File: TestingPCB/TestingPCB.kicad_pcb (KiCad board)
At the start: 2 copper layers, 15 parts, among them J1 Conn_01x04, J2 USB_C_Receptacle_USB2.0_14P, J3 Conn_01x08, U1 SC0915, U2 CP2102N-Axx-xQFN24, U3 USBLC6-2P6

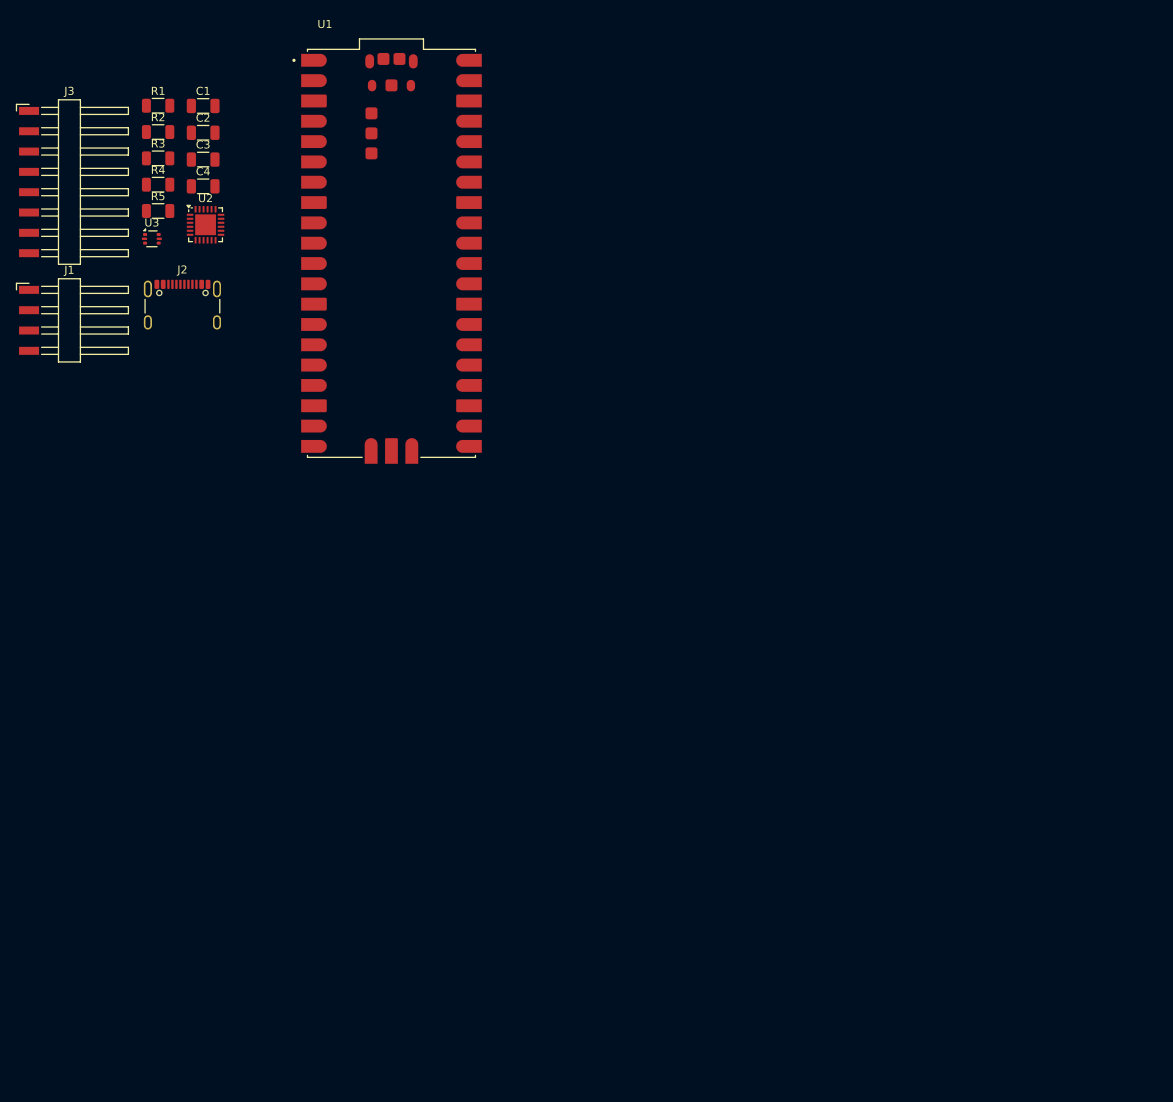
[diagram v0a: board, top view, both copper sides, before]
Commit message: v1 of PCB
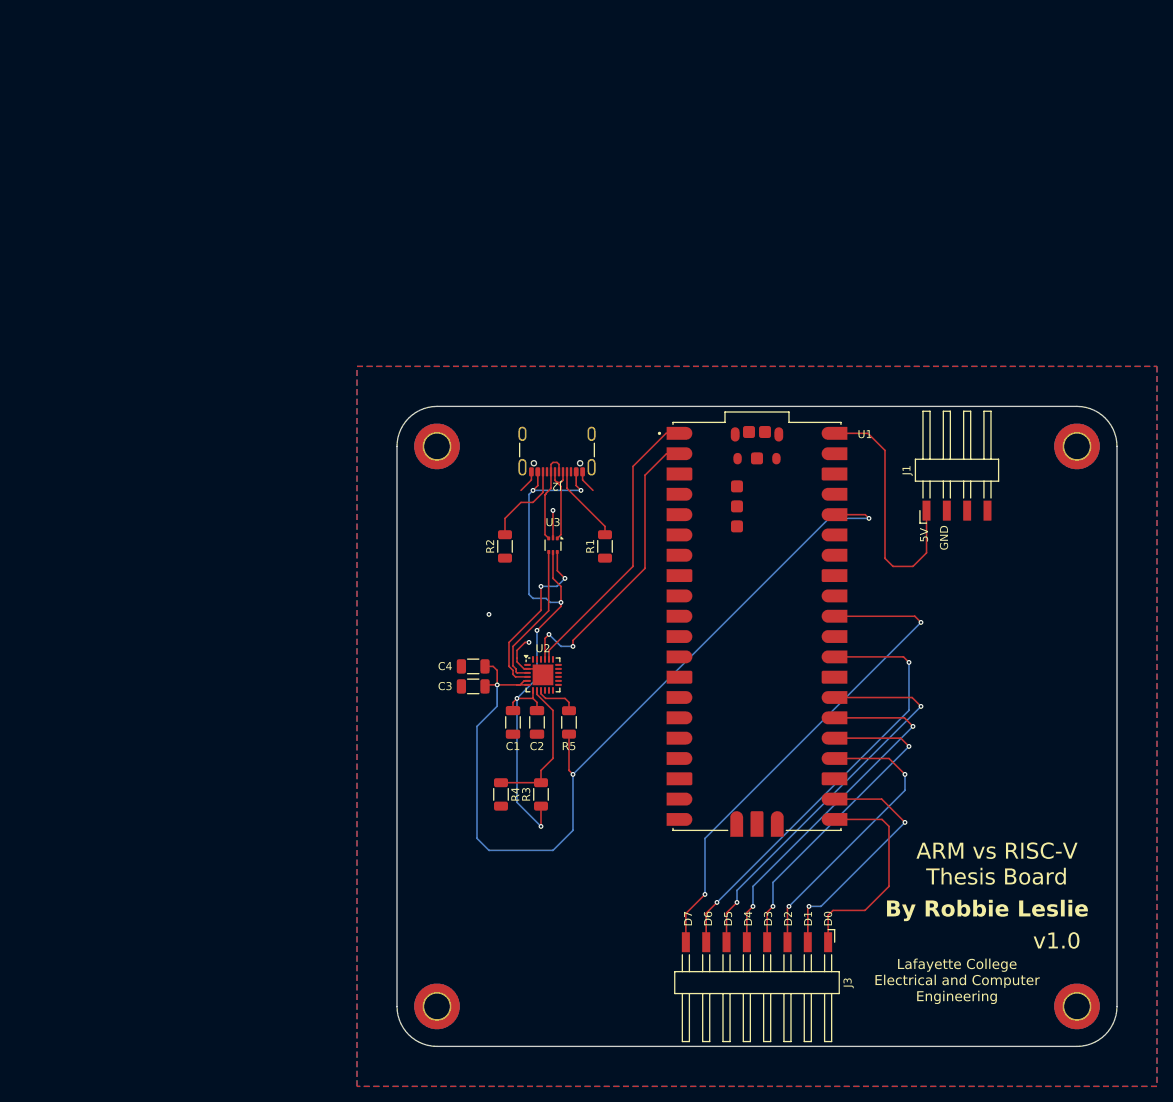
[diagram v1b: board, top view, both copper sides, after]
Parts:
- added H1: MountingHole, MountingHole:MountingHole_3.2mm_M3_ISO7380_Pad_TopBottom, F.Cu at (95.0, 70.0)
- added H2: MountingHole, MountingHole:MountingHole_3.2mm_M3_ISO7380_Pad_TopBottom, F.Cu at (175.0, 70.0)
- added H3: MountingHole, MountingHole:MountingHole_3.2mm_M3_ISO7380_Pad_TopBottom, F.Cu at (95.0, 140.0)
- added H4: MountingHole, MountingHole:MountingHole_3.2mm_M3_ISO7380_Pad_TopBottom, F.Cu at (175.0, 140.0)
- moved J3 132.0 mm to (135.0, 137.5), turned to -90 degrees
- moved J1 112.0 mm to (160.0, 72.5), turned to 90 degrees
- moved R3 92.8 mm to (108.0, 113.5), turned to 90 degrees
- moved R4 87.4 mm to (103.0, 113.5), turned to -90 degrees
- moved C1 86.2 mm to (104.5, 104.5), turned to -90 degrees
- moved C2 84.7 mm to (107.5, 104.5), turned to -90 degrees
- moved R5 82.0 mm to (111.5, 104.5), turned to 90 degrees
- moved R1 78.5 mm to (116.0, 82.5), turned to 90 degrees
- moved C3 74.0 mm to (99.5, 100.0), turned to 180 degrees
- moved U2 70.3 mm to (108.2, 98.6)
- moved C4 68.8 mm to (99.5, 97.5), turned to 180 degrees
- moved R2 67.5 mm to (103.5, 82.5), turned to 90 degrees
- moved U1 65.3 mm to (135.0, 92.5)
- moved U3 63.1 mm to (109.5, 82.3), turned to -90 degrees
- moved J2 49.5 mm to (110.0, 69.5), turned to 180 degrees
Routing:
- net /3.3V: track 0.00 -> 111.3 mm, vias 0 -> 3
- net /USB 5V: track 0.00 -> 75.9 mm, vias 0 -> 6
- net /D7: track 0.00 -> 63.3 mm, vias 0 -> 2
- net /D6: track 0.00 -> 55.1 mm, vias 0 -> 2
- net /D5: track 0.00 -> 50.8 mm, vias 0 -> 2
- net /D4: track 0.00 -> 45.8 mm, vias 0 -> 2
- net /D3: track 0.00 -> 41.6 mm, vias 0 -> 2
- net /RX: track 0.00 -> 37.5 mm, vias 0 -> 2
- net /D2: track 0.00 -> 36.7 mm, vias 0 -> 2
- net /TX: track 0.00 -> 36.0 mm
- net /5V: track 0.00 -> 32.3 mm
- net /D1: track 0.00 -> 30.9 mm, vias 0 -> 2
- net /D0: track 0.00 -> 27.1 mm
- net /D_N: track 0.00 -> 21.9 mm, vias 0 -> 2
- net /D_P: track 0.00 -> 18.5 mm
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- added copper zone on B.Cu, net /GND
- added copper zone on F.Cu, net /GND
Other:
- board outline added: 90 x 80 mm
- board text added: "5V"
- board text added: "ARM vs RISC-V Thesis Board"
- board text added: "By Robbie Leslie"
- board text added: "D0"
- board text added: "D1"
- board text added: "D2"
- board text added: "D3"
- board text added: "D4"
- board text added: "D5"
- board text added: "D6"
- board text added: "D7"
- board text added: "GND"
- board text added: "Lafayette College Electrical and Computer Engineering"
- board text added: "v1.0"
